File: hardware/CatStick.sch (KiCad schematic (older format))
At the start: 77 parts, among them J1 Conn_01x06_Female, J2 Antenna, J4 JTAG, P1 USB_C_Plug_USB2.0, U1 CC1352R1F3RGZR, U2 AP2112K-3.3, U3 RFSW8006QTR7, U4 0900FM15D0039, U5 0900PC15A0036, U6 SW409, U7 ATSAMD21E18A, U8 SX1262IMLTRT, Y1 32.768kHz, Y2 48MHz, Y3 32Mhz_10pF_10ppm

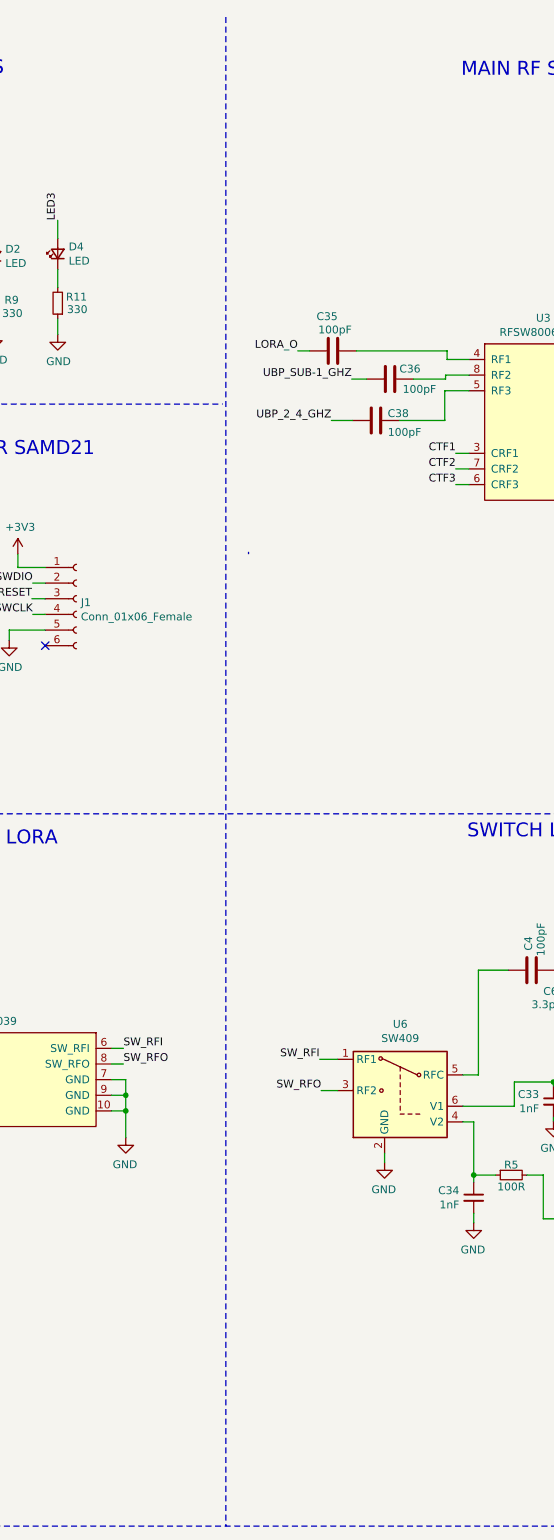
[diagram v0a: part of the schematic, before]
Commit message: fixCrossSignals
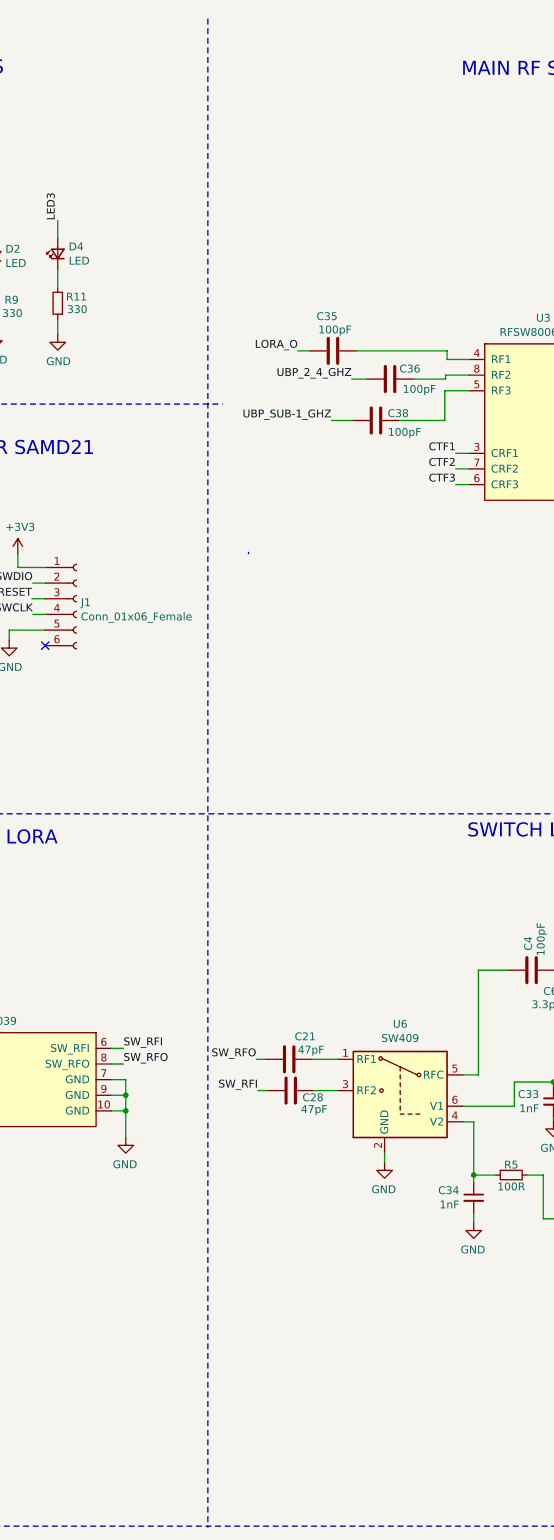
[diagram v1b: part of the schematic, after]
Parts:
- added C21, C28: 47pF, Capacitor_SMD:C_0603_1608Metric, symbol Device:C
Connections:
- net SW_RFI: now also C28.1; no longer U6.1 (RF1)
- net SW_RFO: now also C21.1; no longer U6.3 (RF2)
- net UBP_2_4_GHZ: now also C36.1; no longer C38.1
- net UBP_SUB-1_GHZ: now also C38.1; no longer C36.1
- new net: C21.2, U6.1 (RF1)
- new net: C28.2, U6.3 (RF2)
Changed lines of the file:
@@
 Text Label 20425 3460 2    50   ~ 0
 CTF3
+Text Label 19760 2785 2    50   ~ 0
+UBP_2_4_GHZ
 Text Label 19630 3050 2    50   ~ 0
-UBP_2_4_GHZ
-Text Label 19760 2785 2    50   ~ 0
 UBP_SUB-1_GHZ
 $Comp
@@
 	20470 7235 20570 7235
 Wire Wire Line
-	19670 7135 19555 7135
-Wire Wire Line
-	19670 7335 19565 7335
-Wire Wire Line
 	19970 7735 19970 7795
 $Comp
@@
 	-1   0    0    -1
 $EndComp
-Text Label 19565 7335 2    50   ~ 0
+Text Label 19150 7135 2    50   ~ 0
 SW_RFO
-Text Label 19555 7135 2    50   ~ 0
+Text Label 19160 7335 2    50   ~ 0
 SW_RFI
 Text Label 14670 4205 0    50   ~ 0
@@
 	11945 1865 11945 1995
 Wire Notes Line
-	18955 470  18955 10120
+	18840 480  18840 10130
 $Comp
 L Connector:Conn_01x06_Female J1
@@
 LEDS
 $Comp
-L power:+3V3 #PWR?
+L power:+3V3 #PWR01
 U 1 1 60C1A6B6
 P 1450 4015
-F 0 "#PWR?" H 1450 3865 50  0001 C CNN
+F 0 "#PWR01" H 1450 3865 50  0001 C CNN
 F 1 "+3V3" H 1465 4188 50  0000 C CNN
 F 2 "" H 1450 4015 50  0001 C CNN
@@
 $EndComp
 $Comp
-L power:+3V3 #PWR?
+L power:+3V3 #PWR02
 U 1 1 60C1D5F0
 P 7385 8475
-F 0 "#PWR?" H 7385 8325 50  0001 C CNN
+F 0 "#PWR02" H 7385 8325 50  0001 C CNN
 F 1 "+3V3" H 7400 8648 50  0000 C CNN
 F 2 "" H 7385 8475 50  0001 C CNN
@@
 	1    0    0    -1
 $EndComp
+$Comp
+L Device:C C21
+U 1 1 60977A2F
+P 19360 7135
+F 0 "C21" V 19505 6965 50  0000 L CNN
+F 1 "47pF" V 19420 6910 50  0000 L CNN
+F 2 "Capacitor_SMD:C_0603_1608Metric" H 19398 6985 50  0001 C CNN
+F 3 "" H 19360 7135 50  0000 C CNN
+F 4 "LCSC" H 19360 7135 50  0001 C CNN "provedor"
+F 5 "C14858" H 19360 7135 50  0001 C CNN "LCSC#"
+F 6 "CL10C101JB8NNNC" H 19360 7135 50  0001 C CNN "manf#"
+	1    19360 7135
+	0    -1   -1   0
+$EndComp
+$Comp
+L Device:C C28
+U 1 1 60977E80
+P 19370 7335
+F 0 "C28" V 19325 7125 50  0000 L CNN
+F 1 "47pF" V 19250 7100 50  0000 L CNN
+F 2 "Capacitor_SMD:C_0603_1608Metric" H 19408 7185 50  0001 C CNN
+F 3 "" H 19370 7335 50  0000 C CNN
+F 4 "LCSC" H 19370 7335 50  0001 C CNN "provedor"
+F 5 "C14858" H 19370 7335 50  0001 C CNN "LCSC#"
+F 6 "CL10C101JB8NNNC" H 19370 7335 50  0001 C CNN "manf#"
+	1    19370 7335
+	0    -1   -1   0
+$EndComp
+Wire Wire Line
+	19520 7335 19670 7335
+Wire Wire Line
+	19160 7335 19220 7335
+Wire Wire Line
+	19510 7135 19670 7135
+Wire Wire Line
+	19150 7135 19210 7135
 $EndSCHEMATC
